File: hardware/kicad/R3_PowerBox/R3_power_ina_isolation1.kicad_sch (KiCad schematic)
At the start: 9 parts, among them U6 RS3-0505D/H3

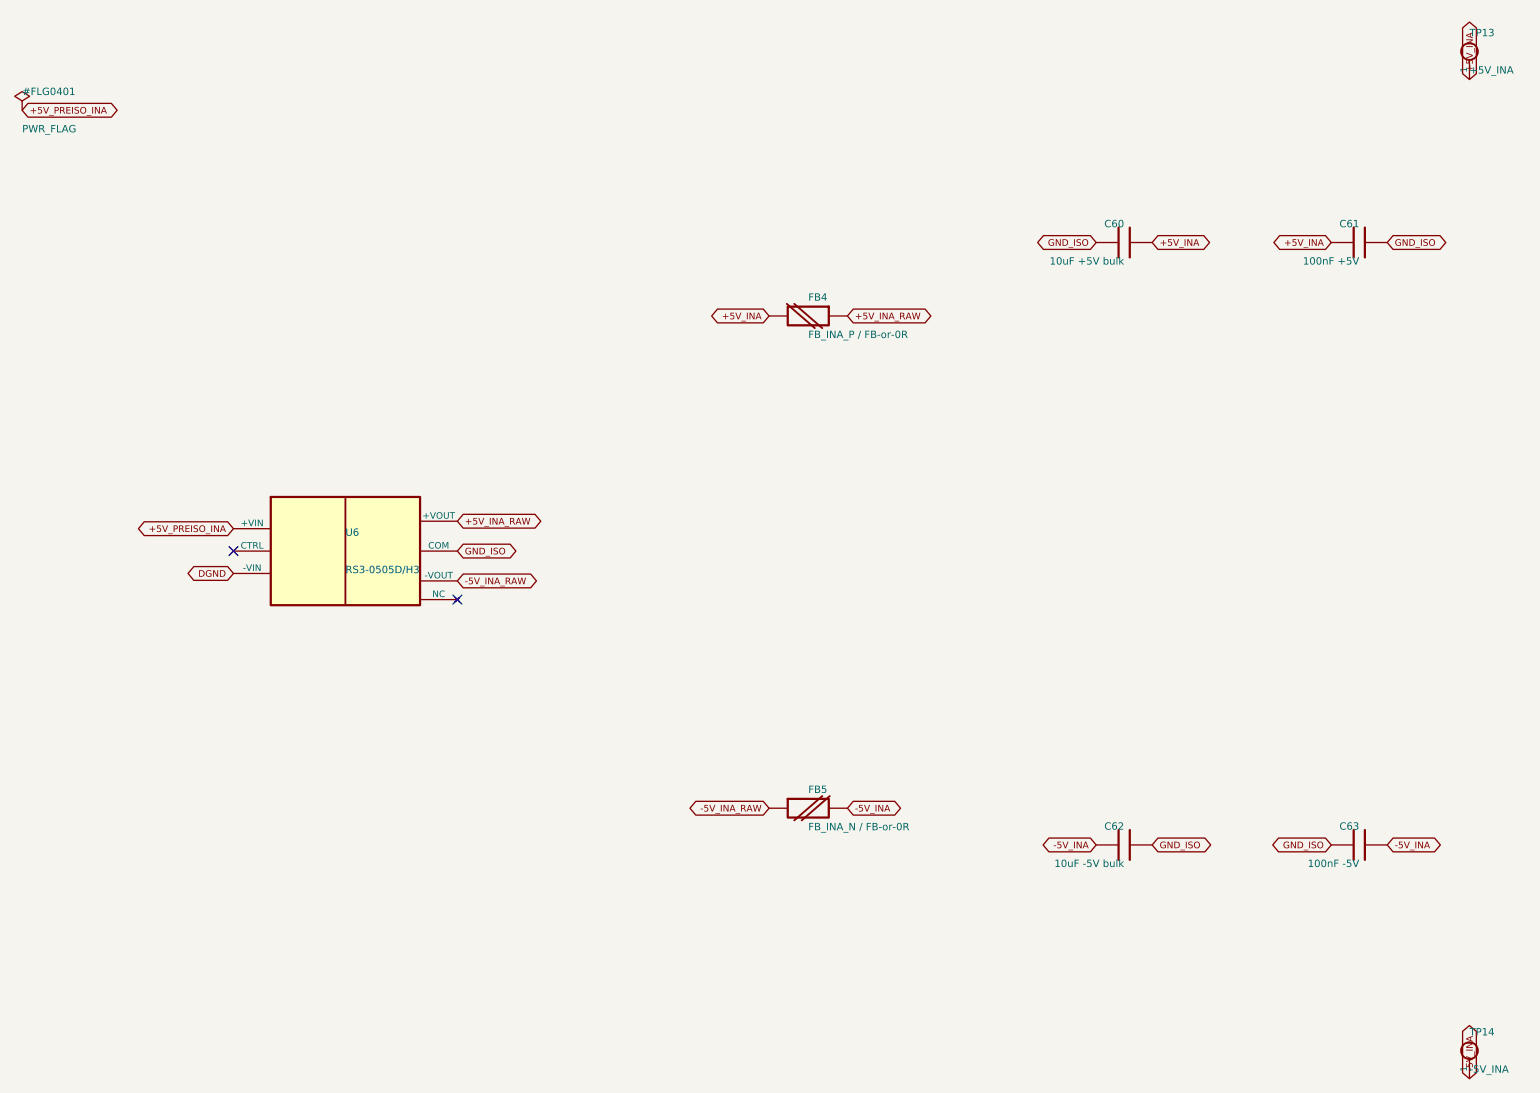
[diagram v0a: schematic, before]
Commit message: Finalize R3 PowerBox pre-placement corrections
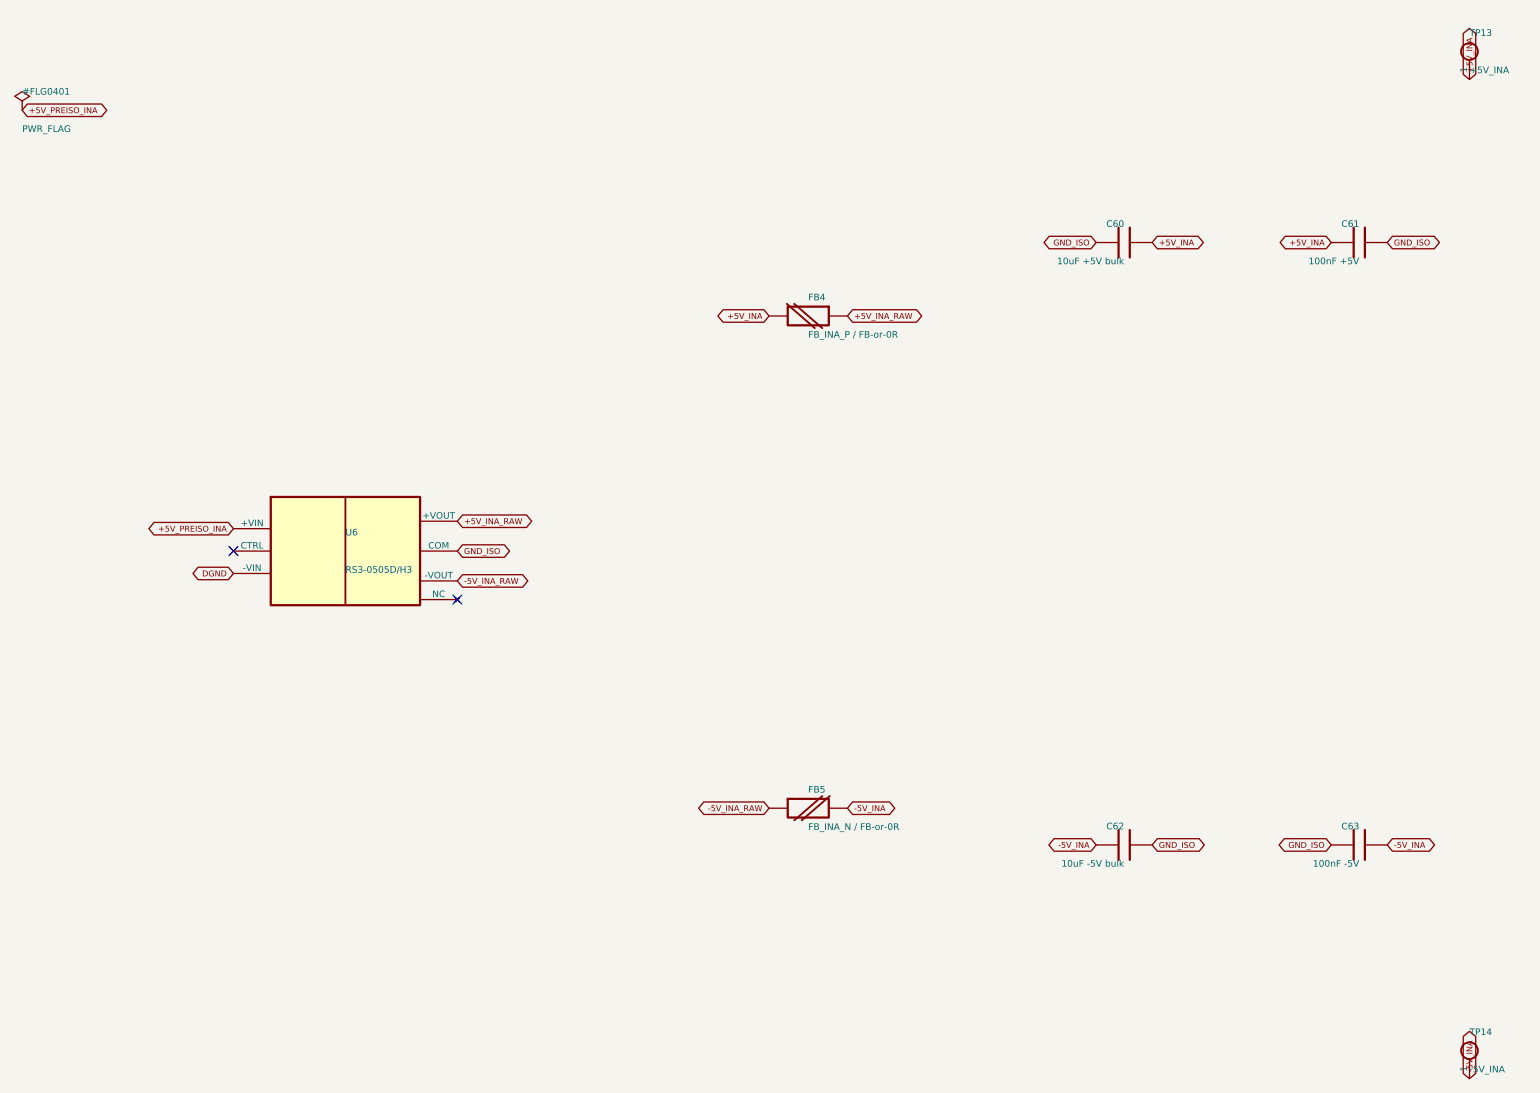
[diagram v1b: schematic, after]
